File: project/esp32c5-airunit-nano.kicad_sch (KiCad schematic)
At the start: 2 parts, among them J1 Conn_01x24_MountingPin, U1 ESP32-C5-WROOM-1U

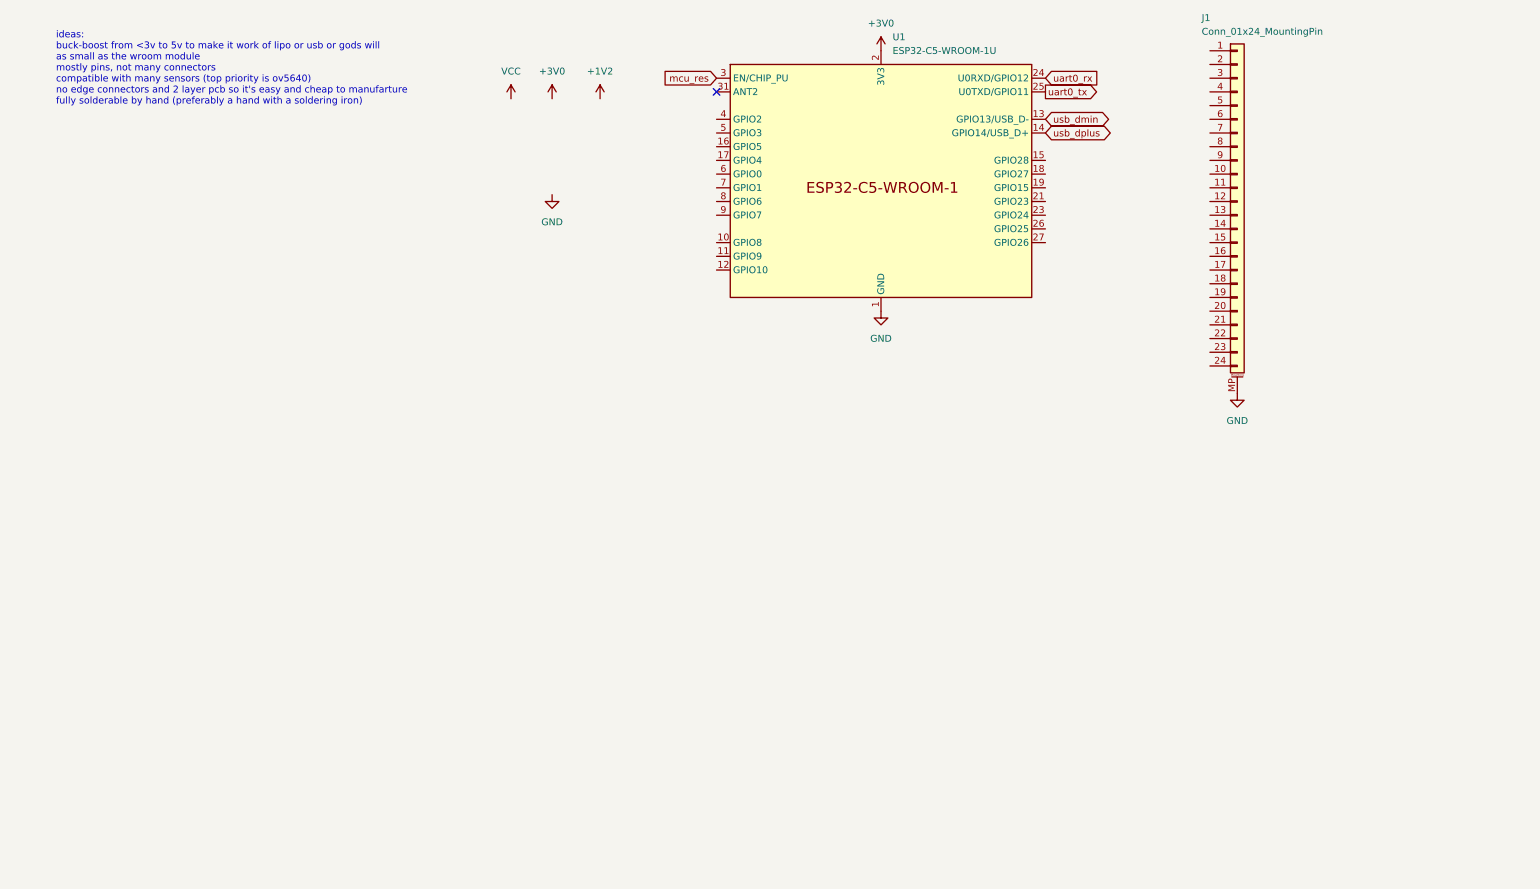
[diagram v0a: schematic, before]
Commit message: i've updated the project files
! ! ! STILL UNFINISHED ! ! !
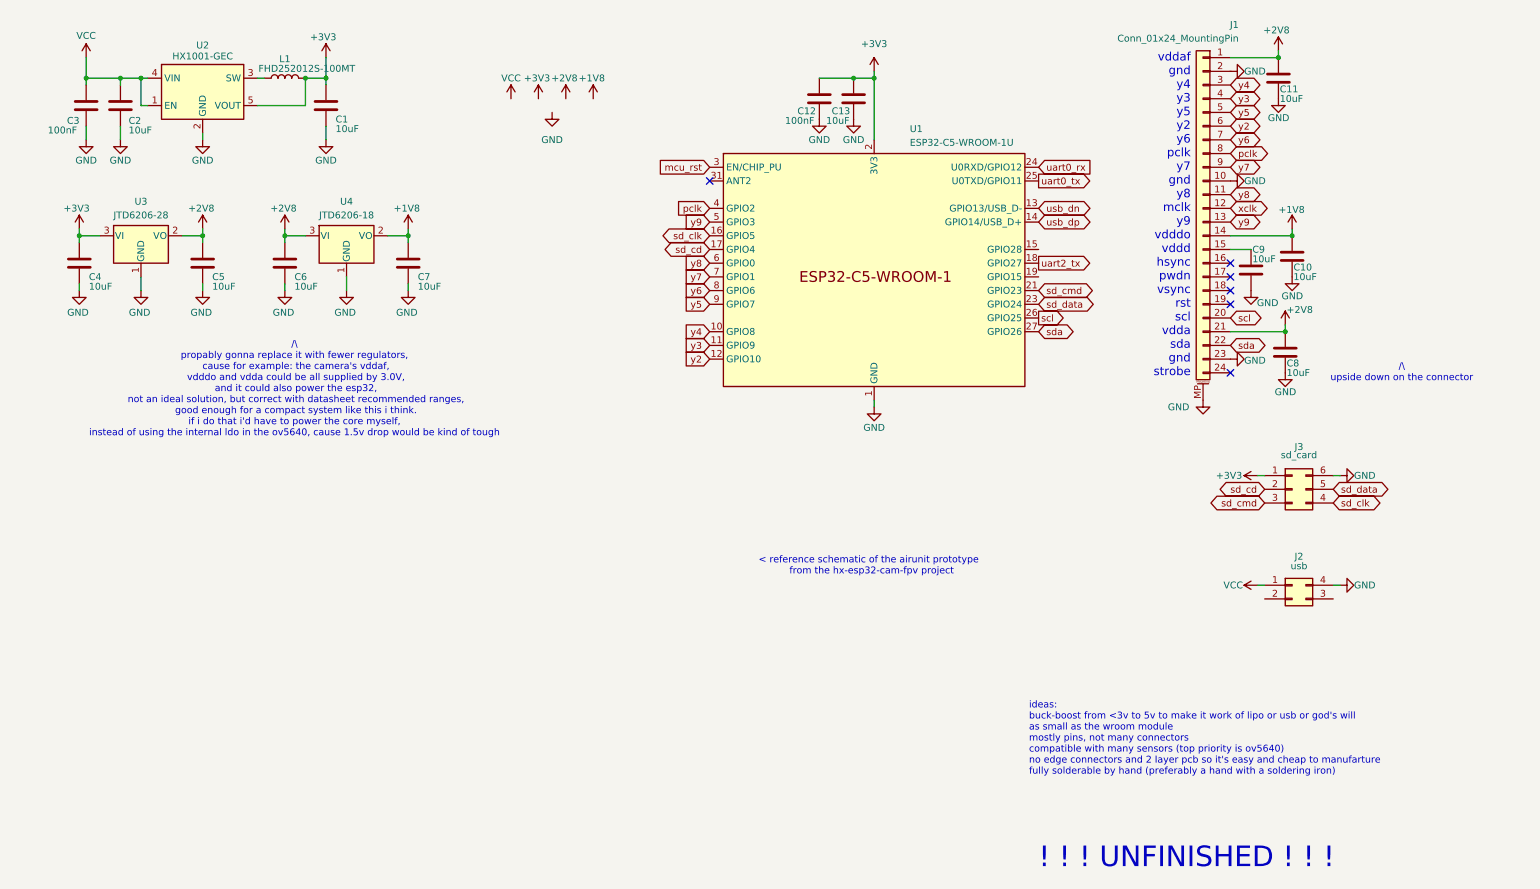
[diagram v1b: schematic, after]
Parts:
- added C1, C10, C11, C13, C2, C4, C5, C6, C7, C8, C9: 10uF, Capacitor_SMD:C_0603_1608Metric, symbol Device:C
- added C12, C3: 100nF, Capacitor_SMD:C_0603_1608Metric, symbol Device:C
- added J2: usb, Connector_PinHeader_1.27mm:PinHeader_2x02_P1.27mm_Vertical, symbol Connector_Generic:Conn_02x02_Counter_Clockwise
- added J3: sd_card, Connector_PinHeader_1.27mm:PinHeader_2x03_P1.27mm_Vertical, symbol Connector_Generic:Conn_02x03_Counter_Clockwise
- added L1: FHD252012S-100MT, Inductor_SMD:L_Changjiang_FNR252010S, symbol Device:L
- added U2: HX1001-GEC, Package_TO_SOT_SMD:TSOT-23-5, symbol Regulator_Switching:PAM2301CAAB330
- added U3: JTD6206-28, Package_TO_SOT_SMD:SOT-23, symbol Regulator_Linear:MCP1700x-280xxTT
- added U4: JTD6206-18, Package_TO_SOT_SMD:SOT-23, symbol Regulator_Linear:MCP1700x-280xxTT
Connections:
- net GND: now also J1.10 (Pin_10), J1.2 (Pin_2), J1.23 (Pin_23), C1.2, C10.1, C11.1, C12.2, C13.2, C2.2, C3.2, C4.2, C5.2, C6.2, C7.2, C8.2, C9.2, J2.4 (Pin_4), J3.6 (Pin_6), U2.2 (GND), U3.1 (GND), U4.1 (GND)
- net VCC: now also C2.1, C3.1, J2.1 (Pin_1), U2.1 (EN), U2.4 (VIN)
- net y4: now reaches U1.10 (GPIO8)
- net y4: now also J1.3 (Pin_3)
- net y3: now reaches U1.11 (GPIO9)
- net y3: now also J1.4 (Pin_4)
- net y2: now reaches U1.12 (GPIO10)
- net y2: now also J1.6 (Pin_6)
- net sd_clk: now reaches U1.16 (GPIO5)
- net sd_clk: now also J3.4 (Pin_4)
- net sd_cd: now reaches U1.17 (GPIO4)
- net sd_cd: now also J3.2 (Pin_2)
- net uart2_tx: now reaches U1.18 (GPIO27)
- net sd_cmd: now reaches U1.21 (GPIO23)
- net sd_cmd: now also J3.3 (Pin_3)
- net sd_data: now reaches U1.23 (GPIO24)
- net sd_data: now also J3.5 (Pin_5)
- net scl: now reaches U1.26 (GPIO25)
- net scl: now also J1.20 (Pin_20)
- net sda: now reaches U1.27 (GPIO26)
- net sda: now also J1.22 (Pin_22)
- net pclk: now reaches U1.4 (GPIO2)
- net pclk: now also J1.8 (Pin_8)
- net y9: now reaches U1.5 (GPIO3)
- net y9: now also J1.13 (Pin_13)
- net y8: now reaches U1.6 (GPIO0)
- net y8: now also J1.11 (Pin_11)
- net y7: now reaches U1.7 (GPIO1)
- net y7: now also J1.9 (Pin_9)
- net y6: now reaches U1.8 (GPIO6)
- net y6: now also J1.7 (Pin_7)
- net y5: now reaches U1.9 (GPIO7)
- net y5: now also J1.5 (Pin_5)
- net +2V8: now reaches J1.1 (Pin_1)
- net +2V8: now also J1.21 (Pin_21), C11.2, C5.1, C6.1, C8.1, U3.2 (VO), U4.3 (VI)
- net xclk: now reaches J1.12 (Pin_12)
- net +1V8: now reaches J1.14 (Pin_14)
- net +1V8: now also C10.2, C7.1, U4.2 (VO)
- net at J1.15 (Pin_15): now also C9.1
- net +3V0 renamed +3V3
- net +3V3: now also C1.1, C12.1, C13.1, C4.1, J3.1 (Pin_1), L1.2, U2.5 (VOUT), U3.3 (VI)
- net mcu_res renamed mcu_rst
- net usb_dmin renamed usb_dn
- net usb_dplus renamed usb_dp
- new net: L1.1, U2.3 (SW)
- no-connect marks 1 -> 6
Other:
- note added: "! ! ! UNFINISHED ! ! !"
- note added: "/\ propably gonna replace it with fewer regulators, cause for example: the camera's vddaf, vdddo and vdda could be all supplied by 3.0V, and it could also power the esp32, not an ideal solution, but correct with datasheet recommended ranges, good enough for a compact system like this i think. if i do that i'd have to power the core myself, instead of using the internal ldo in the ov5640, cause 1.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"
- note added: "/\ upside down on the connector"
- note added: "< reference schematic of the airunit prototype from the hx-esp32-cam-fpv project"
- note added: "ideas: buck-boost from <3v to 5v to make it work of lipo or usb or god's will as small as the wroom module mostly pins, not many connectors compatible with many sensors (top priority is ov5640) no edge connectors and 2 layer pcb so it's easy and cheap to manufarture fully solderable by hand (preferably a hand with a soldering iron)"
- note added: "vddaf gnd y4 y3 y5 y2 y6 pclk y7 gnd y8 mclk y9 vdddo vddd hsync pwdn vsync rst scl vdda sda gnd strobe"
- note removed: "ideas: buck-boost from <3v to 5v to make it work of lipo or usb or gods will as small as the wroom module mostly pins, not many connectors compatible with many sensors (top priority is ov5640) no edge connectors and 2 layer pcb so it's easy and cheap to manufarture fully solderable by hand (preferably a hand with a soldering iron)"
- company: (none) -> us3r_d0e5nt_3x1st
- title: (none) -> esp32c5-airunit-nano
- moved on the sheet: J1, U1

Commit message: i've updated the project files
we're actually getting somewhere, the layout is pretty close to what i would call not bad
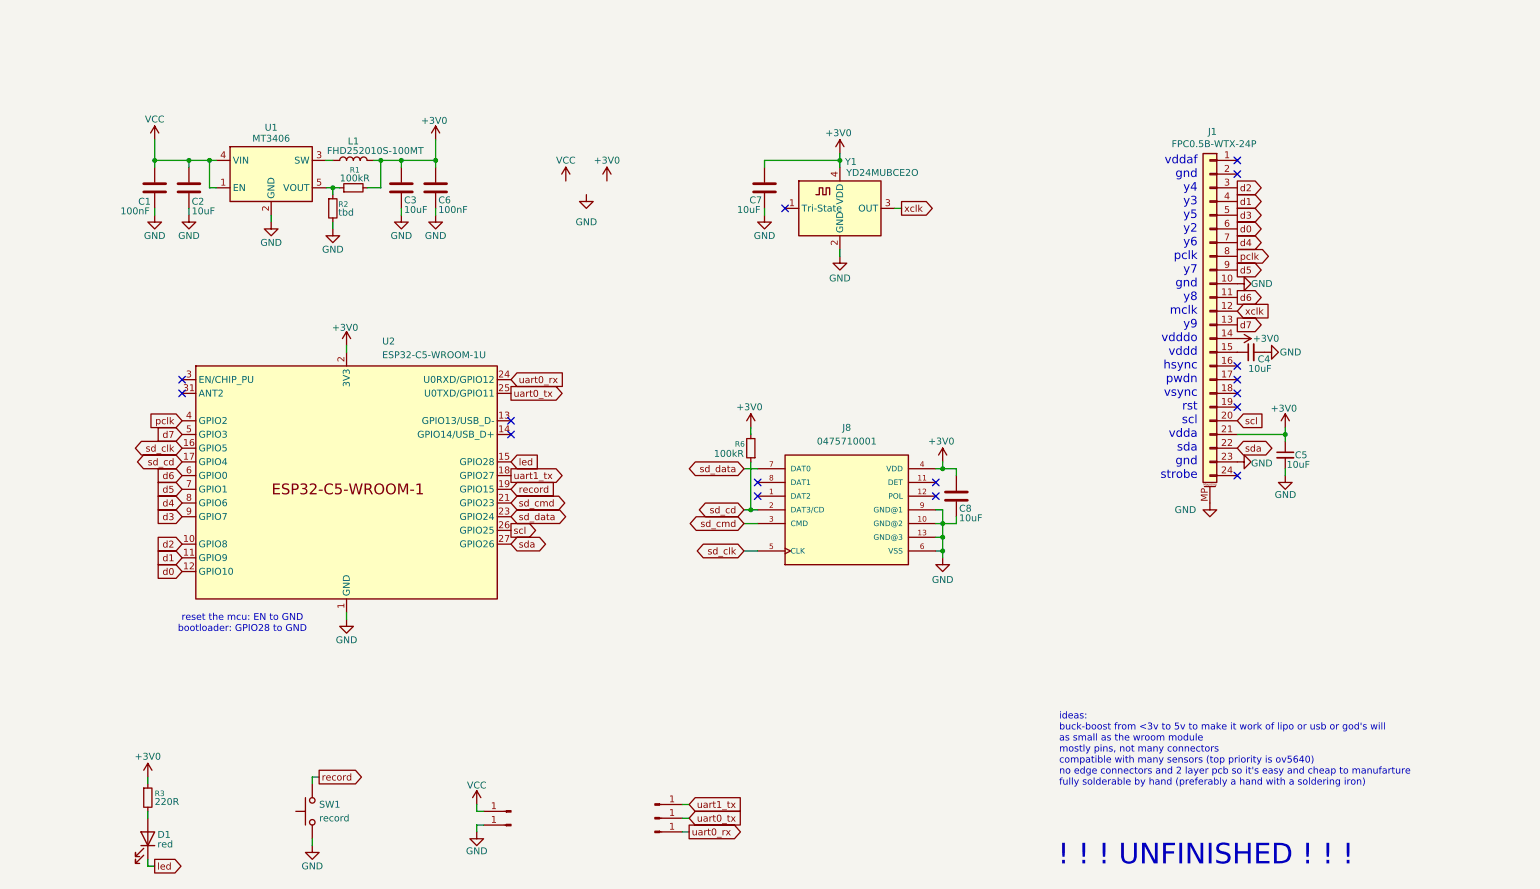
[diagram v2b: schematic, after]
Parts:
- removed C10, C11, C13, C4, C5, C9: 10uF, Capacitor_SMD:C_0603_1608Metric, symbol Device:C
- removed C12: 100nF, Capacitor_SMD:C_0603_1608Metric, symbol Device:C
- removed J2: usb, Connector_PinHeader_1.27mm:PinHeader_2x02_P1.27mm_Vertical, symbol Connector_Generic:Conn_02x02_Counter_Clockwise
- removed J3: sd_card, Connector_PinHeader_1.27mm:PinHeader_2x03_P1.27mm_Vertical, symbol Connector_Generic:Conn_02x03_Counter_Clockwise
- removed U3: JTD6206-28, Package_TO_SOT_SMD:SOT-23, symbol Regulator_Linear:MCP1700x-280xxTT
- removed U4: JTD6206-18, Package_TO_SOT_SMD:SOT-23, symbol Regulator_Linear:MCP1700x-280xxTT
- added C4, C5: 10uF, Capacitor_SMD:C_0603_1608Metric, symbol Device:C_Small
- added D1: red, LED_SMD:LED_0603_1608Metric, symbol Device:LED
- added J2, J4, J5, J6, J7: Conn_01x01_Pin, Library:SolderWirePad_1x01_SMD_2x3mm, symbol Connector:Conn_01x01_Pin
- added J8: 0475710001, 0475710001:MOLEX_0475710001, symbol 0475710001:0475710001
- added R1, R6: 100kR, Resistor_SMD:R_0603_1608Metric, symbol Device:R_Small
- added R2: tbd, Resistor_SMD:R_0603_1608Metric, symbol Device:R_Small
- added R3: 220R, Resistor_SMD:R_0603_1608Metric, symbol Device:R_Small
- added SW1: record, Button_Switch_SMD:SW_SPST_B3U-3000P-B, symbol Switch:SW_Push
- added Y1: YD24MUBCE2O, Oscillator:Oscillator_SMD_ECS_2520MV-xxx-xx-4Pin_2.5x2.0mm, symbol Oscillator:ECS-2520MV-xxx-xx
- C6: value 10uF -> 100nF
- J1: value Conn_01x24_MountingPin -> FPC0.5B-WTX-24P; footprint Connector_FFC-FPC:Hirose_FH12-24S-0.5SH_1x24-1MP_P0.50mm_Horizontal -> Connector_FFC-FPC:TE_2-1734839-4_1x24-1MP_P0.5mm_Horizontal
- L1: value FHD252012S-100MT -> FHD252010S-100MT
- U1: renamed from U2; value HX1001-GEC -> MT3406
- renumbered C3 to C1, C1 to C3, U1 to U2
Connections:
- net GND: now also C4.2, C5.2, J4.1 (Pin_1), J8.10 (GND@2), J8.13 (GND@3), J8.6 (VSS), J8.9 (GND@1), R2.2, SW1.1, Y1.2 (GND); no longer J1.2 (Pin_2)
- net VCC: now also J2.1 (Pin_1)
- net sd_cd: now also J8.2 (DAT3/CD), R6.1
- net sd_clk: now also J8.5 (CLK)
- net sd_cmd: now also J8.3 (CMD)
- net sd_data: now also J8.7 (DAT0)
- net uart0_rx: now also J5.1 (Pin_1)
- net uart0_tx: now also J6.1 (Pin_1)
- net xclk: now also Y1.3 (OUT)
- net at J1.15 (Pin_15): now also C4.1
- net led: now reaches U2.15 (GPIO28)
- net led: now also D1.1 (K)
- net record: now reaches U2.19 (GPIO15)
- net record: now also SW1.2
- net +1V8 renamed +3V0
- net +3V0: now also C3.1, C6.1, C8.1, J1.21 (Pin_21), L1.2, U2.2 (3V3), C5.1, J8.4 (VDD), R1.2, R3.1, R6.2, Y1.4 (VDD)
- removed net +2V8: C6.1, C8.1, J1.1 (Pin_1), J1.21 (Pin_21)
- removed net +3V3: C3.1, L1.2, U1.5 (VOUT), U2.2 (3V3)
- net mcu_rst: no longer names the net of U2.3 (EN/CHIP_PU)
- net uart2_tx renamed uart1_tx
- net uart1_tx: now also J7.1 (Pin_1)
- net usb_dn: no longer names the net of U2.13 (GPIO13/USB_D-)
- net usb_dp: no longer names the net of U2.14 (GPIO14/USB_D+)
- net y2 renamed d0
- net y3 renamed d1
- net y4 renamed d2
- net y5 renamed d3
- net y6 renamed d4
- net y7 renamed d5
- net y8 renamed d6
- net y9 renamed d7
- new net: R1.1, R2.1, U1.5 (VOUT)
- new net: D1.2 (A), R3.2
- no-connect marks 6 -> 16
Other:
- note added: "reset the mcu: EN to GND bootloader: GPIO28 to GND"
- note removed: "/\ propably gonna replace it with fewer regulators, cause for example: the camera's vddaf, vdddo and vdda could be all supplied by 3.0V, and it could also power the esp32, not an ideal solution, but correct with datasheet recommended ranges, good enough for a compact system like this i think. if i do that i'd have to power the core myself, instead of using the internal ldo in the ov5640, cause 1.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"
- note removed: "/\ upside down on the connector"
- note removed: "< reference schematic of the airunit prototype from the hx-esp32-cam-fpv project"
- moved on the sheet: C1, C2, C3, L1, U1, U2

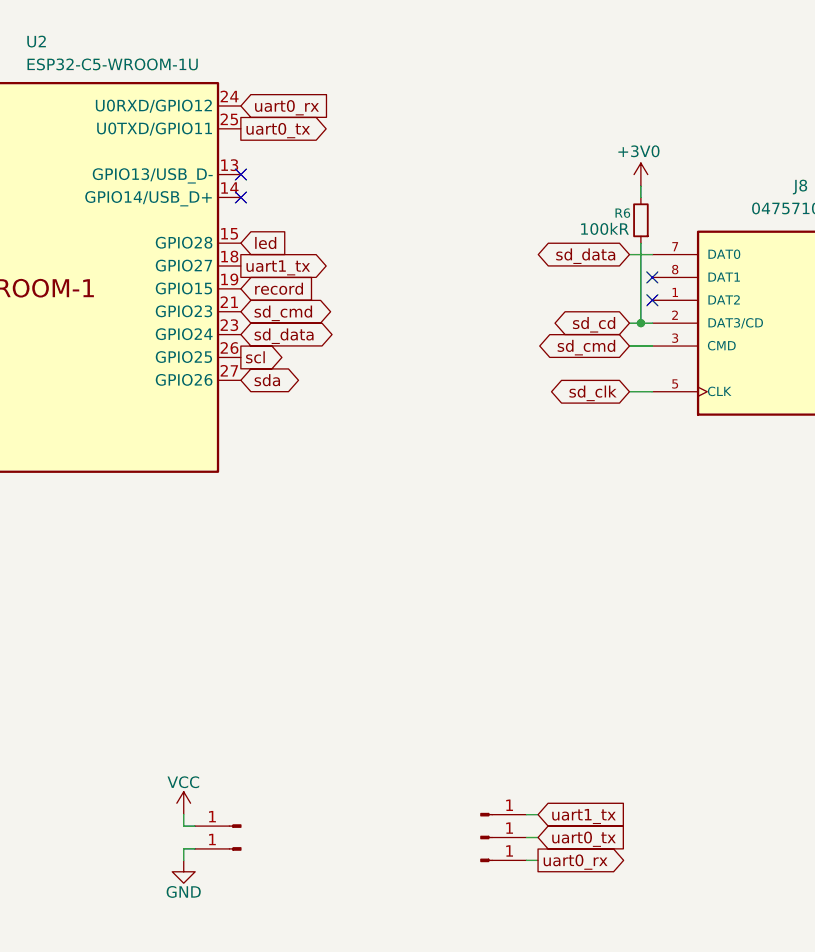
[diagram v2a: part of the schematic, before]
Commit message: Add files via upload
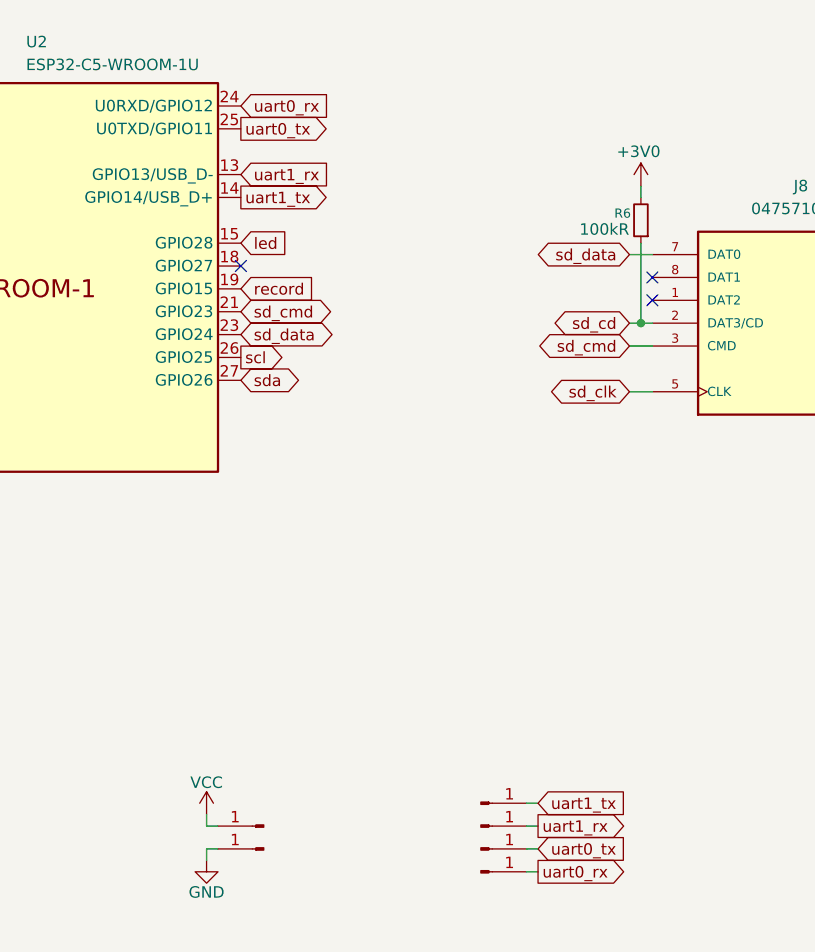
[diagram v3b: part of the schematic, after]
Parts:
- added J9: Conn_01x01_Pin, Library:SolderWirePad_1x01_SMD_2x3mm, symbol Connector:Conn_01x01_Pin
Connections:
- net uart1_tx: now also U2.14 (GPIO14/USB_D+); no longer U2.18 (GPIO27)
- net uart1_rx: now reaches U2.13 (GPIO13/USB_D-)
- net uart1_rx: now also J9.1 (Pin_1)
- no-connect marks 16 -> 15
